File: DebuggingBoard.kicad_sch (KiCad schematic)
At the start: 61 parts, among them J1 Conn_01x05_Socket, J2 Conn_01x08_Socket, J3 Conn_01x01_Socket, SW1 SW_SPDT, U1 STM32F373CCTx, U2 REF5025AD, U3 ADS8866IDRCR, U4 ADG1414BRU, U5 TPS7A4701xRGW, U6 LM27761, U7 LMV358, Y1 16MHz

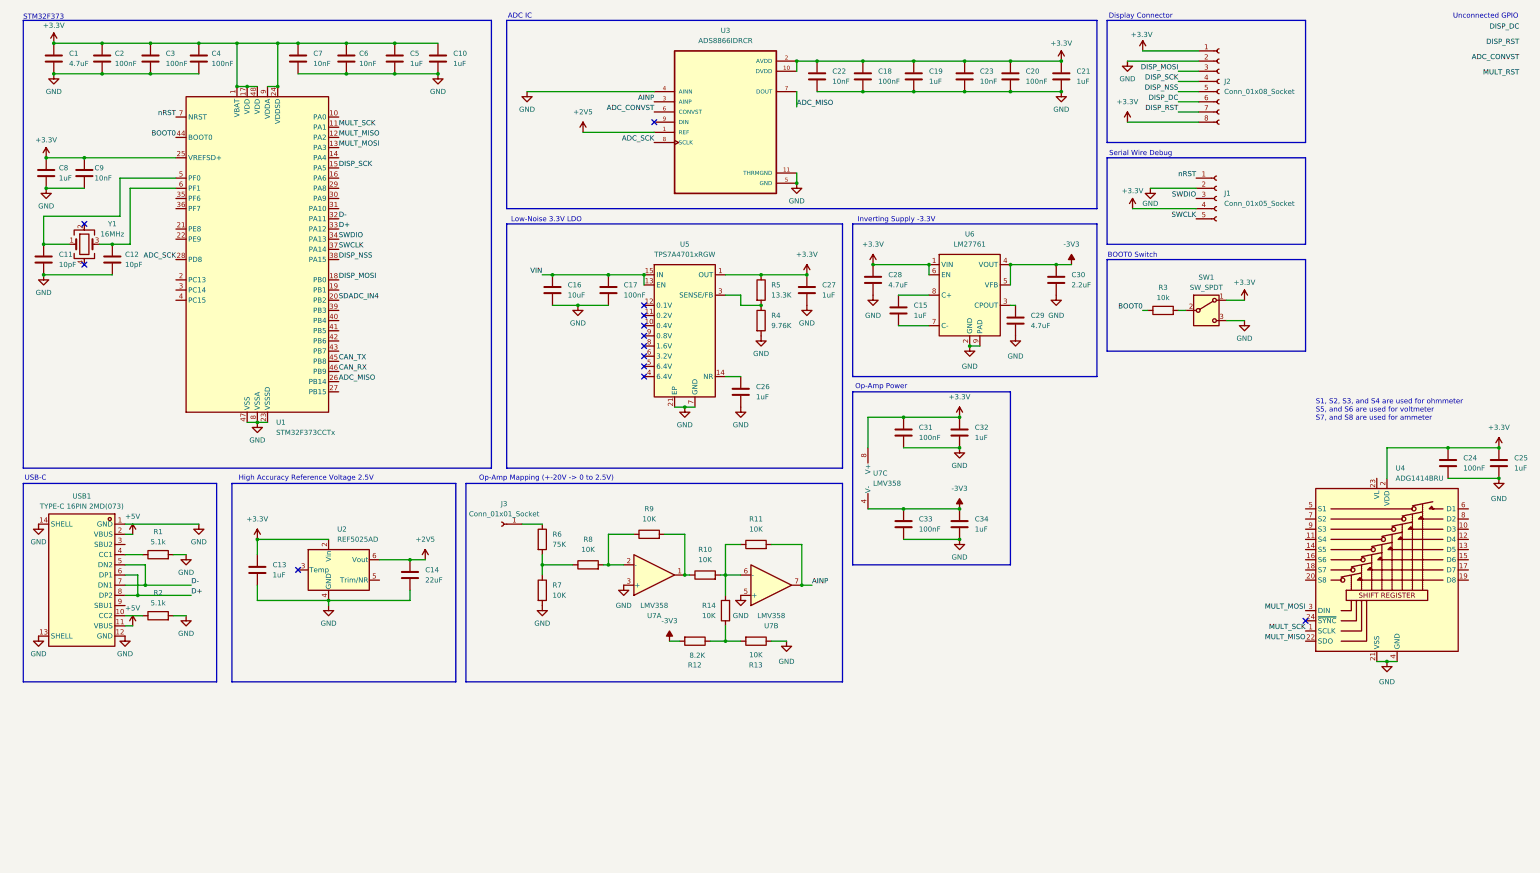
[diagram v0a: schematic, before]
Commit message: nearly final osc
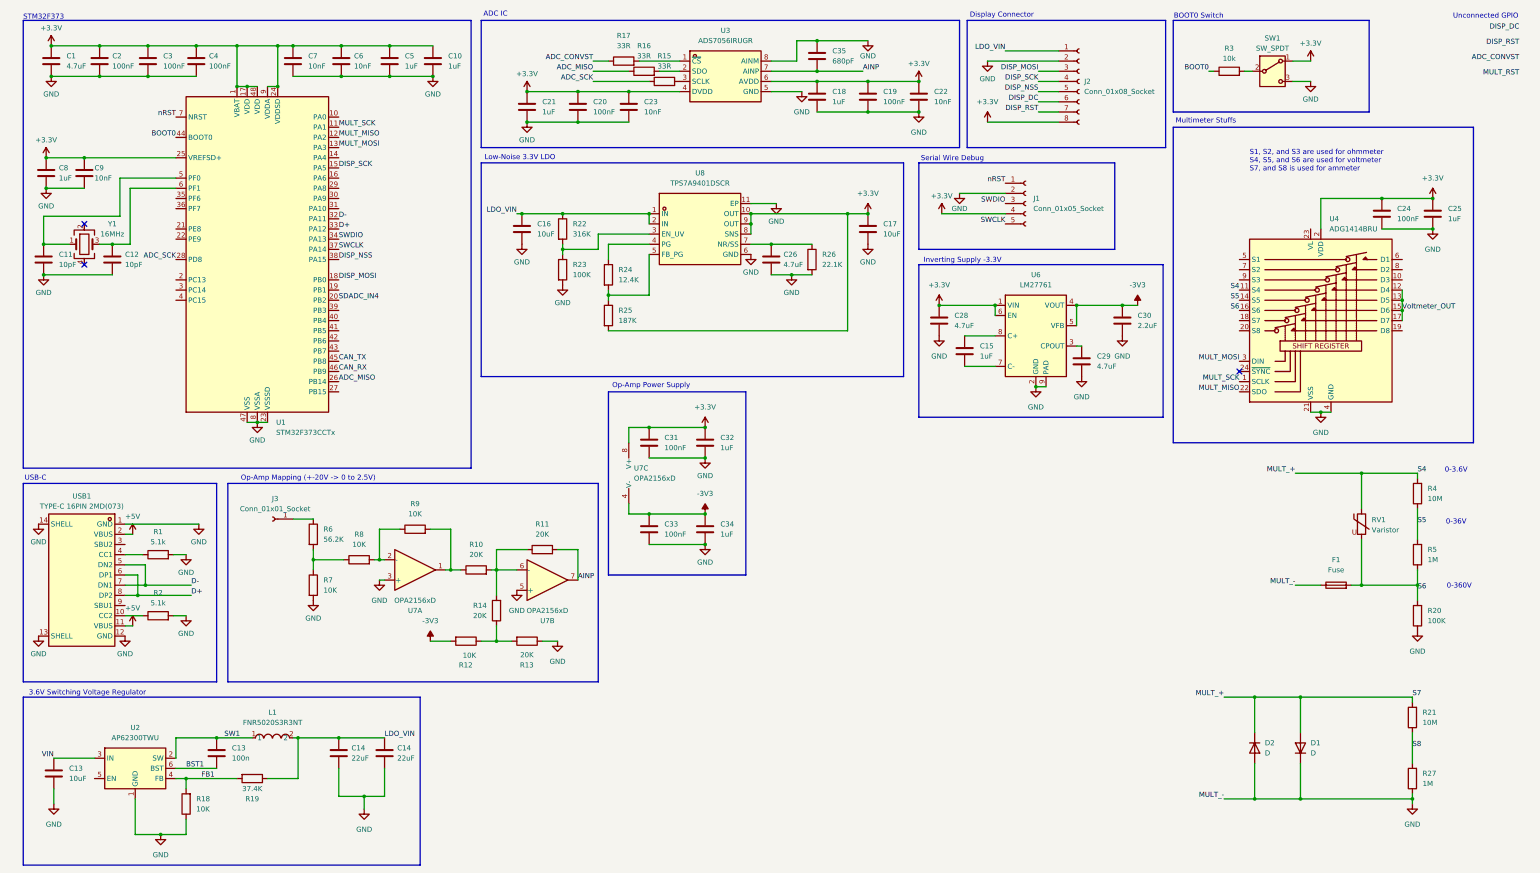
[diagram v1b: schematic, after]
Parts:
- removed C13, C27: 1uF, symbol Device:C
- removed C14: 22uF, symbol Device:C
- removed U2: REF5025AD, Package_SO:SOIC-8_3.9x4.9mm_P1.27mm, symbol Reference_Voltage:REF5025AD
- removed U3: ADS8866IDRCR, ADS8866IDRCR:VREG_V62_16624-01YE, symbol ADS8866:ADS8866IDRCR
- removed U5: TPS7A4701xRGW, Package_DFN_QFN:Texas_RGW0020A_VQFN-20-1EP_5x5mm_P0.65mm_EP3.15x3.15mm_ThermalVias, symbol Regulator_Linear:TPS7A4701xRGW
- removed U7: LMV358, symbol Amplifier_Operational:LMV358
- added C13: 100n, Capacitor_SMD:C_0402_1005Metric, symbol Device:C
- added C13: 10uF, Capacitor_SMD:C_0603_1608Metric, symbol Device:C
- added C14 (x2): 22uF, Capacitor_SMD:C_0805_2012Metric, symbol Device:C
- added C35: 680pF, symbol Device:C
- added D1, D2: D, symbol Device:D
- added F1: Fuse, symbol Device:Fuse
- added L1: FNR5020S3R3NT, Rocketry_Easyeda:IND-SMD_L5.0-W5.0_FNR50XXS, symbol Rocketry:FNR5020S3R3NT
- added R15, R16, R17: 33R, symbol Device:R
- added R18: 10K, Resistor_SMD:R_0402_1005Metric, symbol Device:R
- added R19: 37.4K, Resistor_SMD:R_0402_1005Metric, symbol Device:R
- added R20, R23: 100K, symbol Device:R
- added R21: 10M, symbol Device:R
- added R22: 316K, symbol Device:R
- added R24: 12.4K, symbol Device:R
- added R25: 187K, symbol Device:R
- added R26: 22.1K, symbol Device:R
- added R27: 1M, symbol Device:R
- added RV1: Varistor, symbol Device:Varistor
- added U2: AP62300TWU, Package_TO_SOT_SMD:TSOT-23-6, symbol Regulator_Switching:AP62300TWU
- added U3: ADS7056IRUGR, Rocketry_Easyeda:X2QFN-8_L1.5-W1.5-P0.50-BL, symbol ROCKETRY_EASYEDA:ADS7056IRUGR
- added U7: OPA2156xD, Package_SO:SOIC-8_3.9x4.9mm_P1.27mm, symbol Amplifier_Operational:OPA2156xD
- added U8: TPS7A9401DSCR, Rocketry_Easyeda:WSON-10_L3.0-W3.0-P0.50-TL-EP, symbol ROCKETRY_EASYEDA:TPS7A9401DSCR
- C17: value 100nF -> 10uF
- C18: value 100nF -> 1uF
- C19: value 1uF -> 100nF
- C26: value 1uF -> 4.7uF
- R10, R11, R13, R14: value 10K -> 20K
- R12: value 8.2K -> 10K
- R4: value 9.76K -> 10M
- R5: value 13.3K -> 1M
- R6: value 75K -> 56.2K
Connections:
- net +3.3V: now also C17.1, R25.2, U3.4 (DVDD), U3.6 (AVDD), U7.8 (V+), U8.10 (OUT), U8.8 (SNS), U8.9 (OUT); no longer J2.1 (Pin_1), R5.1
- net -3V3: now also U7.4 (V-)
- net ADC_CONVST: now also R17.1
- net ADC_MISO: now also R16.1
- net ADC_SCK: now also R15.1
- net AINP: now also C35.2, U3.7 (AINP), U7.7
- net GND: now also C13.2, C14.2, C14.2, C35.1, D1.1 (K), D2.2 (A), F1.1, R18.1, R20.1, R23.2, R26.2, R27.1, U2.1 (GND), U3.5 (GND), U3.8 (AINM), U7.3 (+), U7.5 (+), U8.11 (EP), U8.6 (GND); no longer R4.2
- net VIN: now also C13.1, U2.3 (IN); no longer C16.1, C17.1
- net S5: now reaches R4.1, R5.2
- net S5: now also U4.14 (S5)
- net at R10.2, R11.1, R14.2: now also U7.6 (-)
- net at R8.2, R9.1: now also U7.2 (-)
- net at R10.1, R9.2: now also U7.1
- net at C26.1: now also R26.1, U8.7 (NR/SS)
- net MULT_+: now reaches U4.11 (S4)
- net MULT_+: now also R4.2, D1.2 (A), D2.1 (K), R21.2, RV1.1
- net Voltmeter_OUT: now reaches U4.12 (D4)
- net Voltmeter_OUT: now also U4.13 (D5), U4.15 (D6), U4.17 (D7)
- net S6: now reaches U4.16 (S6)
- net S6: now also R5.1, F1.2, R20.2, RV1.2
- new net: R24.2, R25.1, U8.5 (FB_PG)
- new net: R17.2, U3.1 (~{CS})
- new net: R16.2, U3.2 (SDO)
- new net: R15.2, U3.3 (SCLK)
- new net: R22.2, R23.1, U8.3 (EN_UV)
- new net: R24.1, U8.4 (PG)
- new net BST1: C13.1, U2.6 (BST)
- new net FB1: R18.2, R19.2, U2.4 (FB)
- new net LDO_VIN: C14.1, C14.1, C16.1, J2.1 (Pin_1), L1.2, R19.1, R22.1, U8.1 (IN), U8.2 (IN)
- new net S8: R21.1, R27.2
- new net SW1: C13.2, L1.1, U2.2 (SW)
- no-connect marks 13 -> 3
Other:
- note added: "0-3.6V"
- note added: "0-360V"
- note added: "0-36V"
- note added: "3.6V Switching Voltage Regulator"
- note added: "Multimeter Stuffs"
- note added: "Op-Amp Power Supply"
- note added: "S1, S2, and S3 are used for ohmmeter S4, S5, and S6 are used for voltmeter S7, and S8 is used for ammeter"
- note removed: "High Accuracy Reference Voltage 2.5V"
- note removed: "Op-Amp Power"
- note removed: "S1, S2, S3, and S4 are used for ohmmeter S5, and S6 are used for voltmeter S7, and S8 are used for ammeter"
- moved on the sheet: C1, C10, C15, C2, C20, C21, C23, C24, C25, C28, C29, C3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
